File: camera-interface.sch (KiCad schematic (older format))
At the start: 44 parts, among them J8 WE_68715014522, U19 NTS0102GT, U20 NTS0102GT, U22 AP2114H-3_3TRG1

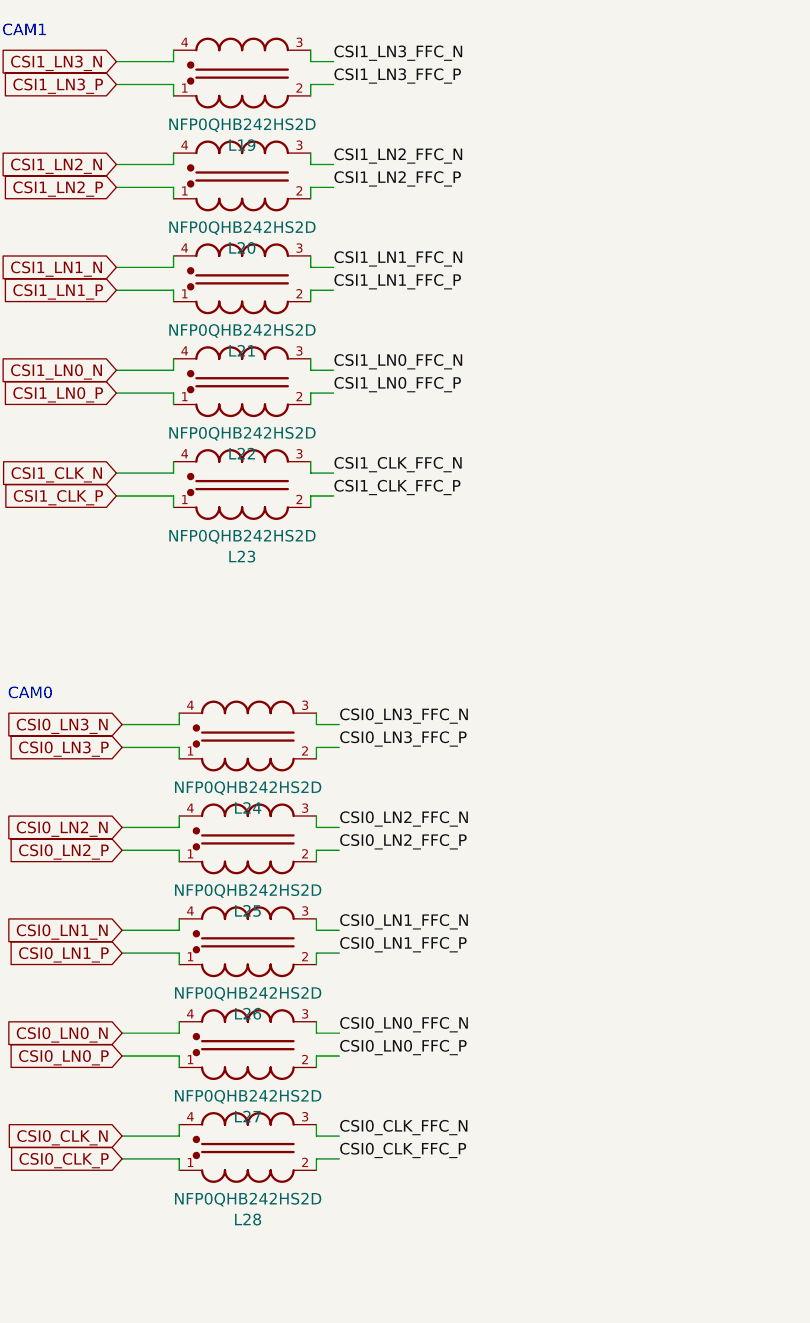
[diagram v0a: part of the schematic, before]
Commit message: Cleanup
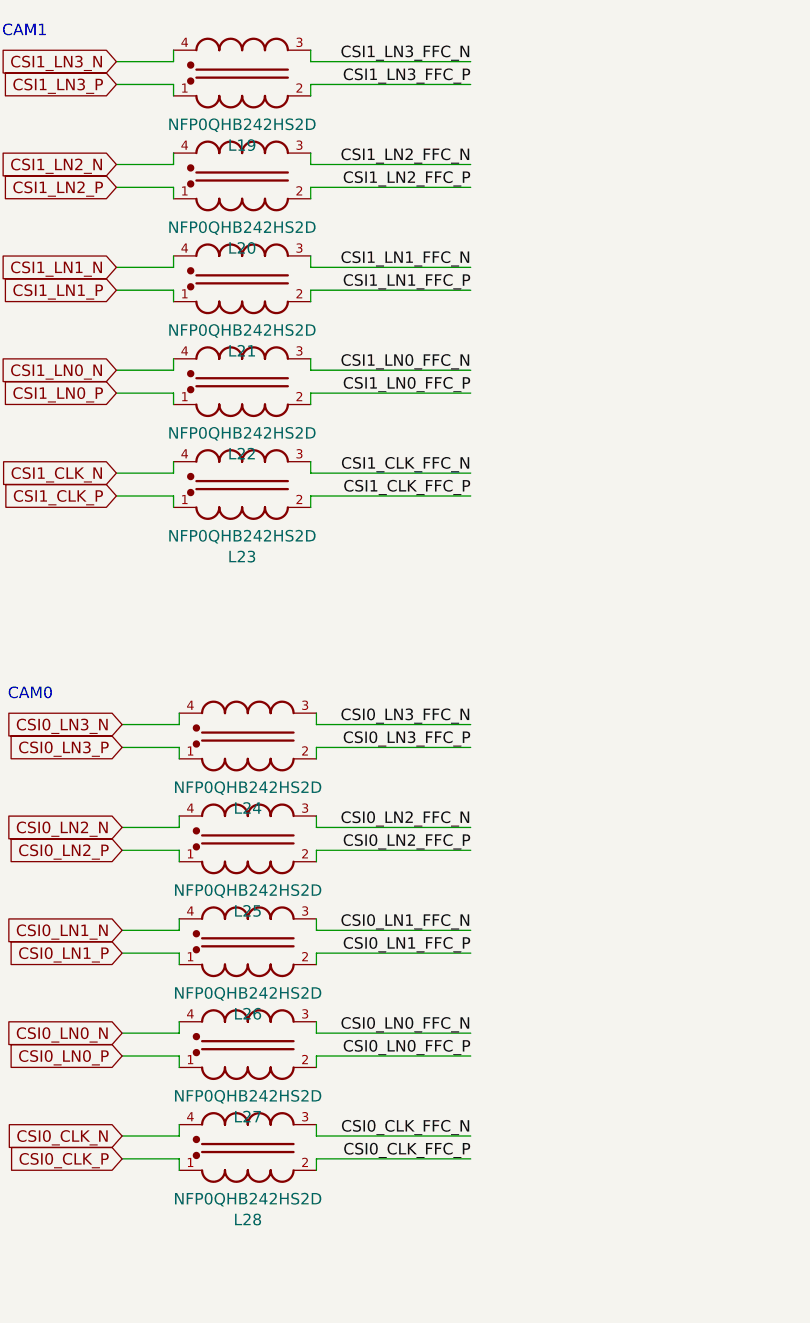
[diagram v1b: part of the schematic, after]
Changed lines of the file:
@@
 $Descr A3 16535 11693
 encoding utf-8
-Sheet 7 13
+Sheet 7 12
 Title ""
 Date ""
@@
 $EndComp
 Wire Wire Line
-	2050 1550 2150 1550
-Wire Wire Line
-	2050 1650 2150 1650
-Text Label 2150 1550 0    50   ~ 0
+	2050 1550 2750 1550
+Wire Wire Line
+	2050 1650 2750 1650
+Text Label 2750 1550 2    50   ~ 0
 CSI1_LN3_FFC_N
-Text Label 2150 1650 0    50   ~ 0
+Text Label 2750 1650 2    50   ~ 0
 CSI1_LN3_FFC_P
 Text Label 6450 1650 0    50   ~ 0
@@
 Text Label 6450 1750 0    50   ~ 0
 CSI1_LN3_FFC_P
-Text Label 2175 4450 0    50   ~ 0
+Text Label 2750 4450 2    50   ~ 0
 CSI0_LN3_FFC_N
-Text Label 2175 4550 0    50   ~ 0
+Text Label 2750 4550 2    50   ~ 0
 CSI0_LN3_FFC_P
 Text Label 6450 3450 0    50   ~ 0
@@
 CSI0_LN3_FFC_P
 Wire Wire Line
-	2075 4450 2175 4450
-Wire Wire Line
-	2075 4550 2175 4550
+	2075 4450 2750 4450
+Wire Wire Line
+	2075 4550 2750 4550
 Wire Wire Line
 	2050 1950 2050 2000
 Wire Wire Line
-	2050 2000 2150 2000
+	2050 2000 2750 2000
 Wire Wire Line
 	2050 2150 2050 2100
 Wire Wire Line
-	2050 2100 2150 2100
+	2050 2100 2750 2100
 Wire Wire Line
 	2050 2400 2050 2450
 Wire Wire Line
-	2050 2450 2150 2450
+	2050 2450 2750 2450
 Wire Wire Line
 	2050 2600 2050 2550
 Wire Wire Line
-	2050 2550 2150 2550
+	2050 2550 2750 2550
 Wire Wire Line
 	2050 2850 2050 2900
 Wire Wire Line
-	2050 2900 2150 2900
+	2050 2900 2750 2900
 Wire Wire Line
 	2050 3050 2050 3000
 Wire Wire Line
-	2050 3000 2150 3000
+	2050 3000 2750 3000
 Wire Wire Line
 	2050 3300 2050 3350
 Wire Wire Line
-	2050 3350 2150 3350
+	2050 3350 2750 3350
 Wire Wire Line
 	2050 3500 2050 3450
 Wire Wire Line
-	2050 3450 2150 3450
-Text Label 2150 2000 0    50   ~ 0
+	2050 3450 2750 3450
+Text Label 2750 2000 2    50   ~ 0
 CSI1_LN2_FFC_N
-Text Label 2150 2100 0    50   ~ 0
+Text Label 2750 2100 2    50   ~ 0
 CSI1_LN2_FFC_P
-Text Label 2150 2550 0    50   ~ 0
+Text Label 2750 2550 2    50   ~ 0
 CSI1_LN1_FFC_P
-Text Label 2150 2450 0    50   ~ 0
+Text Label 2750 2450 2    50   ~ 0
 CSI1_LN1_FFC_N
-Text Label 2150 2900 0    50   ~ 0
+Text Label 2750 2900 2    50   ~ 0
 CSI1_LN0_FFC_N
-Text Label 2150 3000 0    50   ~ 0
+Text Label 2750 3000 2    50   ~ 0
 CSI1_LN0_FFC_P
-Text Label 2150 3350 0    50   ~ 0
+Text Label 2750 3350 2    50   ~ 0
 CSI1_CLK_FFC_N
-Text Label 2150 3450 0    50   ~ 0
+Text Label 2750 3450 2    50   ~ 0
 CSI1_CLK_FFC_P
 Wire Wire Line
 	2075 4850 2075 4900
 Wire Wire Line
-	2075 4900 2175 4900
+	2075 4900 2750 4900
 Wire Wire Line
 	2075 5050 2075 5000
 Wire Wire Line
-	2075 5000 2175 5000
+	2075 5000 2750 5000
 Wire Wire Line
 	2075 5300 2075 5350
 Wire Wire Line
-	2075 5350 2175 5350
+	2075 5350 2750 5350
 Wire Wire Line
 	2075 5500 2075 5450
 Wire Wire Line
-	2075 5450 2175 5450
+	2075 5450 2750 5450
 Wire Wire Line
 	2075 5750 2075 5800
 Wire Wire Line
-	2075 5800 2175 5800
+	2075 5800 2750 5800
 Wire Wire Line
 	2075 5950 2075 5900
 Wire Wire Line
-	2075 5900 2175 5900
+	2075 5900 2750 5900
 Wire Wire Line
 	2075 6200 2075 6250
 Wire Wire Line
-	2075 6250 2175 6250
+	2075 6250 2750 6250
 Wire Wire Line
 	2075 6400 2075 6350
 Wire Wire Line
-	2075 6350 2175 6350
-Text Label 2175 4900 0    50   ~ 0
+	2075 6350 2750 6350
+Text Label 2750 4900 2    50   ~ 0
 CSI0_LN2_FFC_N
-Text Label 2175 5000 0    50   ~ 0
+Text Label 2750 5000 2    50   ~ 0
 CSI0_LN2_FFC_P
-Text Label 2175 5350 0    50   ~ 0
+Text Label 2750 5350 2    50   ~ 0
 CSI0_LN1_FFC_N
-Text Label 2175 5450 0    50   ~ 0
+Text Label 2750 5450 2    50   ~ 0
 CSI0_LN1_FFC_P
-Text Label 2175 5800 0    50   ~ 0
+Text Label 2750 5800 2    50   ~ 0
 CSI0_LN0_FFC_N
-Text Label 2175 5900 0    50   ~ 0
+Text Label 2750 5900 2    50   ~ 0
 CSI0_LN0_FFC_P
-Text Label 2175 6250 0    50   ~ 0
+Text Label 2750 6250 2    50   ~ 0
 CSI0_CLK_FFC_N
-Text Label 2175 6350 0    50   ~ 0
+Text Label 2750 6350 2    50   ~ 0
 CSI0_CLK_FFC_P
 Text Label 6450 1850 0    50   ~ 0
